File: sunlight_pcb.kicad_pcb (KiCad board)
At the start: 2 copper layers, 136.5 x 127 mm, 17 parts, among them J1 Conn_01x01, J2 Conn_01x01, J3 Conn_01x01, J4 Conn_01x01, J8 PJ-002AH, Q1 DMN63D8LW, Q2 DMN63D8LW, U1 LDH-65-700, U2 LDH-65-700, U3 SeeedStudio ESP32-C3, U4 LMTOE78_03-0.5

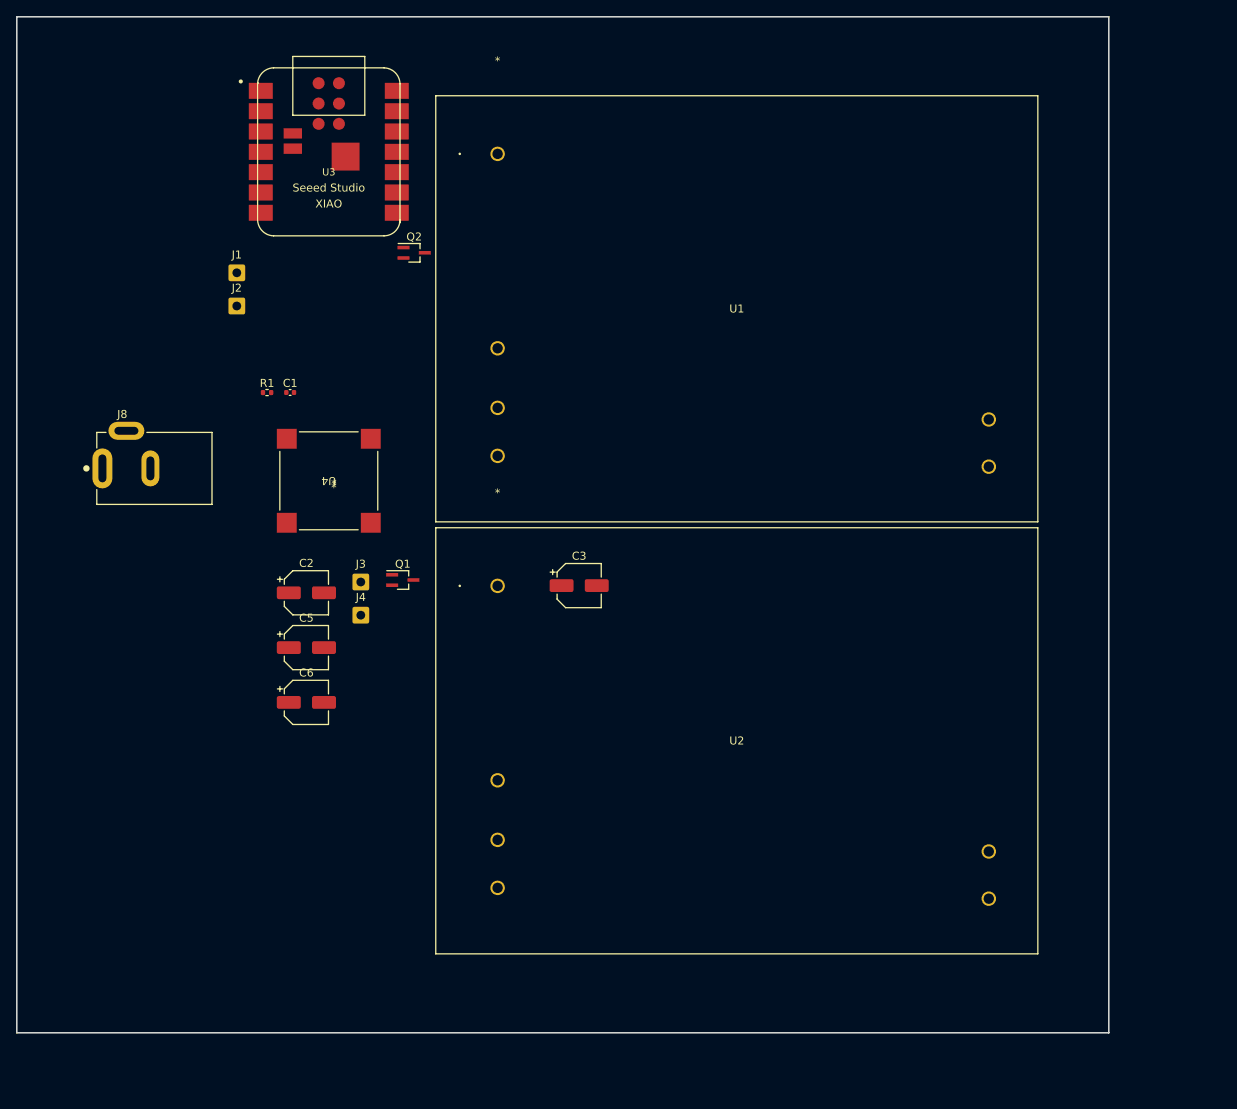
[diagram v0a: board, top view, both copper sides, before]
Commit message: layout done, gerbers gened
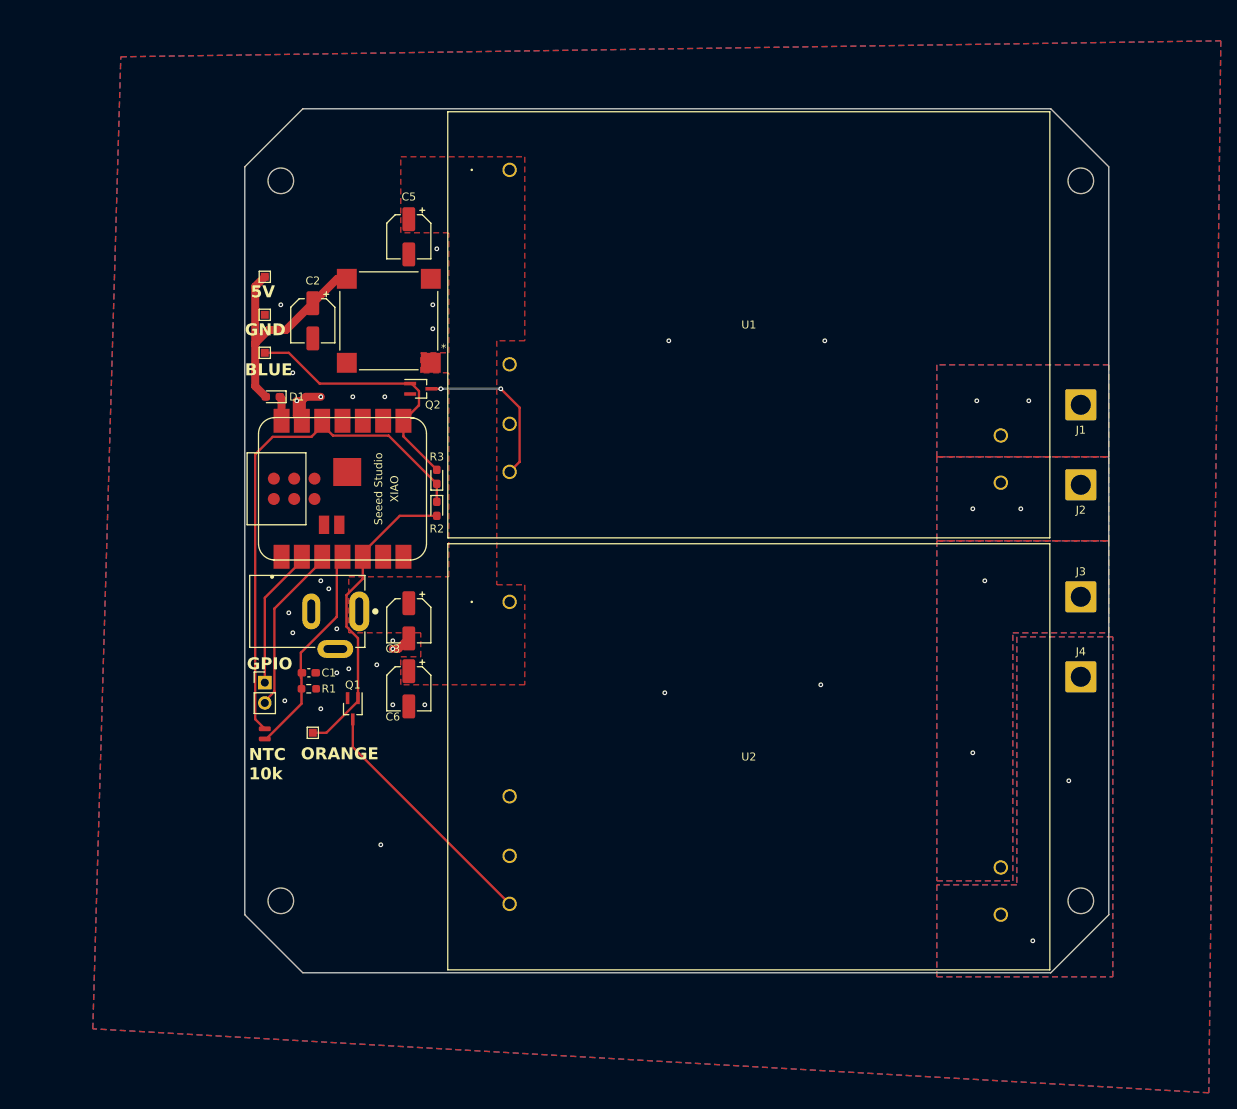
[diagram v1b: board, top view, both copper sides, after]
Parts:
- added D1: D_Schottky, Diode_SMD:D_0603_1608Metric_Pad1.05x0.95mm_HandSolder, F.Cu at (85.5, 72.0)
- added J5: NTC, sunlight_pcb:SolderNTC-1.27mm, F.Cu at (84.5, 113.5)
- added J7: Conn_01x02, Connector_PinHeader_2.54mm:PinHeader_1x02_P2.54mm_Vertical, F.Cu at (84.5, 107.7)
- added R2: 10k, Diode_SMD:D_0603_1608Metric_Pad1.05x0.95mm_HandSolder, F.Cu at (106.0, 86.0)
- added R3: 10k, Diode_SMD:D_0603_1608Metric_Pad1.05x0.95mm_HandSolder, F.Cu at (106.0, 82.0)
- added REF**: MountingHole_3.2mm_M3, MountingHole:MountingHole_3.2mm_M3, F.Cu at (186.5, 135.0)
- added REF**: MountingHole_3.2mm_M3, MountingHole:MountingHole_3.2mm_M3, F.Cu at (186.5, 45.0)
- added REF**: MountingHole_3.2mm_M3, MountingHole:MountingHole_3.2mm_M3, F.Cu at (86.5, 135.0)
- added REF**: MountingHole_3.2mm_M3, MountingHole:MountingHole_3.2mm_M3, F.Cu at (86.5, 45.0)
- added TP1: TestPoint, TestPoint:TestPoint_Pad_1.0x1.0mm, F.Cu at (84.5, 66.5)
- added TP2: TestPoint, TestPoint:TestPoint_Pad_1.0x1.0mm, F.Cu at (90.5, 114.0)
- added TP3: TestPoint, TestPoint:TestPoint_Pad_1.0x1.0mm, F.Cu at (84.5, 57.0)
- added TP4: TestPoint, TestPoint:TestPoint_Pad_1.0x1.0mm, F.Cu at (84.5, 61.8)
- C1: footprint Capacitor_SMD:C_0402_1005Metric -> Capacitor_SMD:C_0603_1608Metric_Pad1.08x0.95mm_HandSolder
- J1, J2, J3, J4: footprint Connector_Wire:SolderWire-0.5sqmm_1x01_D0.9mm_OD2.1mm -> Connector_Wire:SolderWire-2sqmm_1x01_D2mm_OD3.9mm
- R1: footprint Resistor_SMD:R_0402_1005Metric -> Resistor_SMD:R_0603_1608Metric_Pad0.98x0.95mm_HandSolder
- moved J2 107.8 mm to (186.5, 83.0), turned to 180 degrees
- moved J1 106.8 mm to (186.5, 73.0), turned to 180 degrees
- moved J4 90.3 mm to (186.5, 107.0)
- moved J3 90.0 mm to (186.5, 97.0)
- moved C5 52.9 mm to (102.5, 52.0), turned to -90 degrees
- moved U3 42.2 mm to (94.2, 83.5), turned to 90 degrees
- moved R1 37.4 mm to (90.0, 108.5), turned to 180 degrees
- moved J8 36.8 mm to (96.3, 98.8), turned to 180 degrees
- moved C1 35.1 mm to (90.0, 106.5)
- moved C2 34.0 mm to (90.5, 62.5), turned to -90 degrees
- moved C3 21.7 mm to (102.5, 100.0), turned to -90 degrees
- moved U4 21.4 mm to (100.0, 62.5)
- moved Q1 17.3 mm to (95.5, 111.0), turned to -90 degrees
- moved Q2 17.0 mm to (104.0, 71.0)
- moved C6 12.9 mm to (102.5, 108.5), turned to -90 degrees
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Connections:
- J8 pad 3: unconnected-(J8-Pad3) -> GND
- U3 pad 1: Net-(J5-Pin_2) -> unconnected-(U3-PA02_A0_D0-Pad1)
- U3 pad 12: unconnected-(U3-3V3-Pad12) -> +3V3
- U3 pad 2: unconnected-(U3-PA4_A1_D1-Pad2) -> /UART_RX
- U3 pad 3: unconnected-(U3-PA10_A2_D2-Pad3) -> /UART_TX
- U3 pad 4: unconnected-(U3-PA11_A3_D3-Pad4) -> Net-(J5-Pin_2)
- U3 pad 6: /BLUE_INPUT -> unconnected-(U3-PA9_A5_D5_SCL-Pad6)
- U3 pad 7: /UART_TX -> unconnected-(U3-PB08_A6_D6_TX-Pad7)
- U3 pad 8: /UART_RX -> /BLUE_INPUT
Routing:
- net +3V3: track 0.00 -> 65.4 mm
- net /ORANGE_INPUT: track 0.00 -> 38.4 mm
- net /BLUE_INPUT: track 0.00 -> 33.6 mm
- net Net-(Q1-D): track 0.00 -> 31.2 mm
- net +5V: track 0.00 -> 31.0 mm
- net Net-(J5-Pin_2): track 0.00 -> 27.1 mm
- net /UART_TX: track 0.00 -> 21.0 mm
- net Net-(Q2-D): track 0.00 -> 20.5 mm, vias 0 -> 2
- net /UART_RX: track 0.00 -> 17.4 mm
- net GND: track 0.00 -> 10.4 mm, vias 0 -> 28
- net Net-(D1-K): track 0.00 -> 3.09 mm
- net Net-(J4-Pin_1): vias 0 -> 2
- net Net-(J3-Pin_1): vias 0 -> 2
- net Net-(J2-Pin_1): vias 0 -> 2
- net Net-(J1-Pin_1): vias 0 -> 2
- added copper zone on F.Cu, net +24V
- added copper zone on B.Cu, net GND
- added copper zone on F.Cu, net GND
- added copper zone on B.Cu, net Net-(J1-Pin_1)
- added copper zone on F.Cu, net Net-(J1-Pin_1)
- added copper zone on B.Cu, net Net-(J2-Pin_1)
- added copper zone on F.Cu, net Net-(J2-Pin_1)
- added copper zone on B.Cu, net Net-(J3-Pin_1)
- added copper zone on F.Cu, net Net-(J3-Pin_1)
- added copper zone on B.Cu, net Net-(J4-Pin_1)
- added copper zone on F.Cu, net Net-(J4-Pin_1)
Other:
- board size 136.5 x 127 mm -> 108 x 108 mm
- board text added: "5V"
- board text added: "BLUE"
- board text added: "GND"
- board text added: "GPIO"
- board text added: "NTC 10k"
- board text added: "ORANGE"
